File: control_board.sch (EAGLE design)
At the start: 19 parts

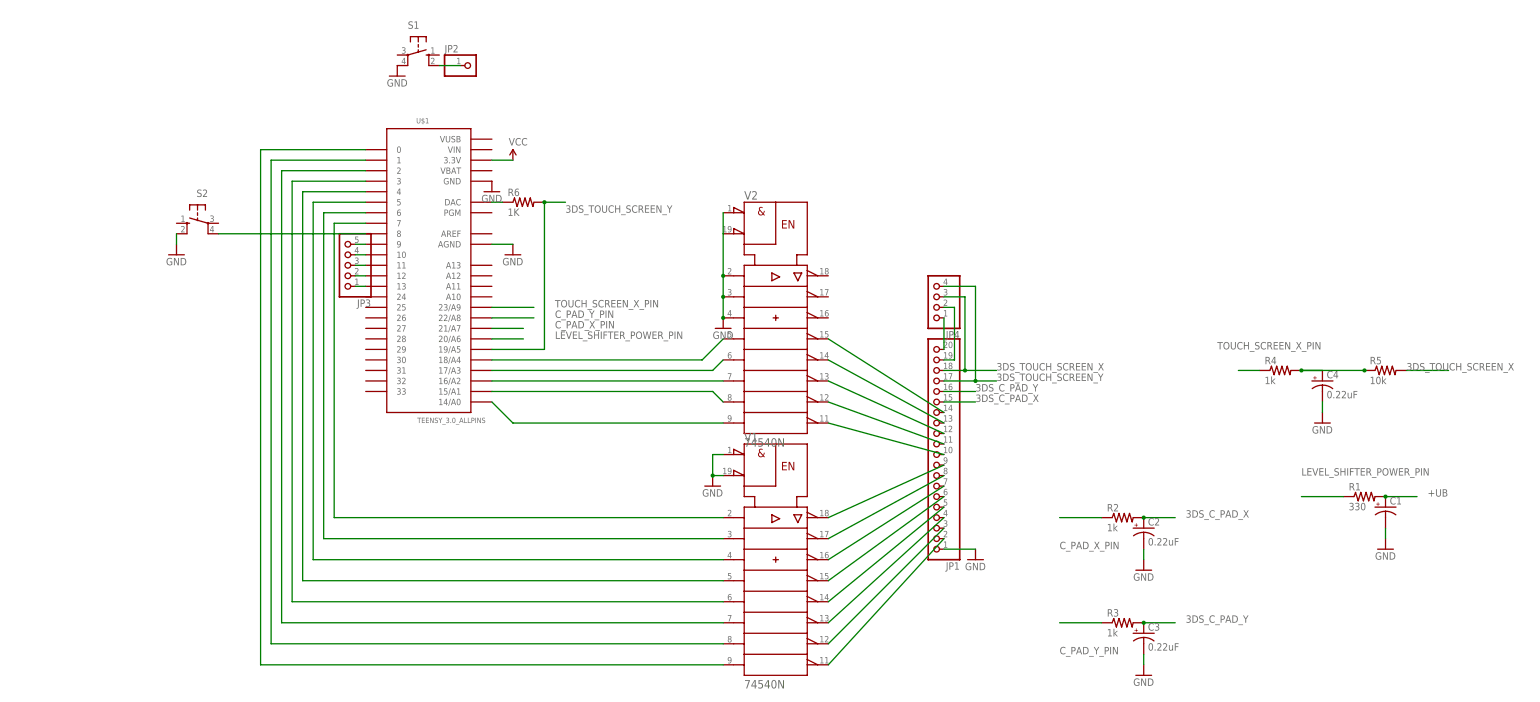
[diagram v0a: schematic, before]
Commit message: First commit
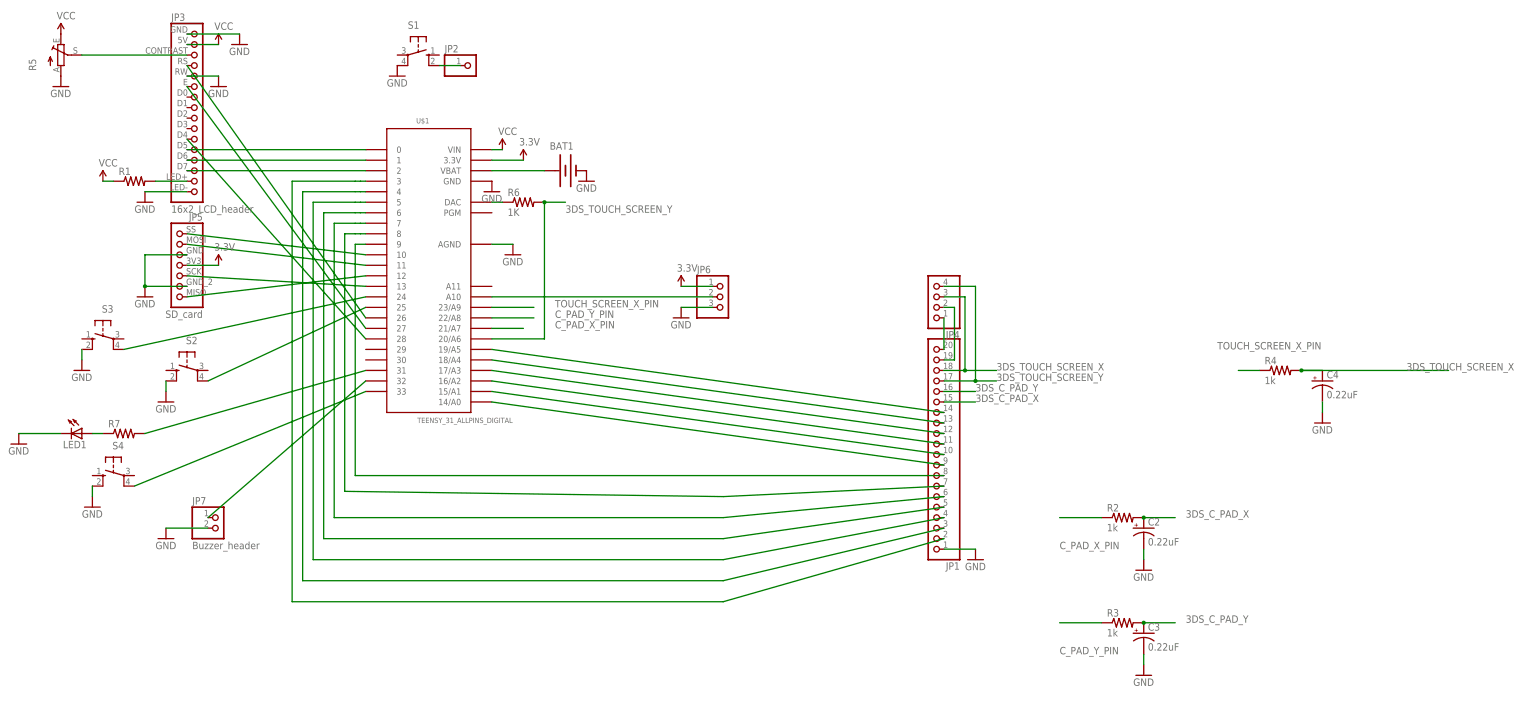
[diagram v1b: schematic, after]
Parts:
- removed C1: (no value), SparkFun-Capacitors:10UF-25V-20%(PTH)
- removed V1, V2: 74540N, 74ttl-din:74540N
- added BAT1: (no value), SparkFun-Electromechanical:BATTERY20PTH
- added JP5: SD_card, sd_header:PINHD-1X7
- added JP6: (no value), pinhead:PINHD-1X3
- added JP7: Buzzer_header, pinhead:PINHD-1X2
- added LED1: (no value), adafruit:LED5MM
- added R7: (no value), SparkFun-Resistors:RESISTOREZ
- added S3, S4: (no value), switch-omron:10-XX
- JP3: value (none) -> 16x2_LCD_header; device pinhead:PINHD-1X5 -> LCD_HEADER:PINHD-1X16
- R1: value 330 -> (none); device resistor:R-US_0207/7 -> SparkFun-Resistors:RESISTOREZ
- R2, R3, R4: device resistor:R-US_0207/7 -> SparkFun-Resistors:RESISTORPTH-1/4W-VERT
- R5: value 10k -> (none); device SparkFun-Resistors:RESISTORPTH-1/4W-VERT -> pot:TRIM_EU-CA6V
- R6: device rcl:R-US_0207/7 -> SparkFun-Resistors:RESISTORPTH-1/4W-VERT
- U$1: value TEENSY_3.0_ALLPINS -> TEENSY_31_ALLPINS_DIGITAL; device Teensy3.0:TEENSY_3.0_ALLPINS -> Teensy3.0:TEENSY_31_ALLPINS_DIGITAL
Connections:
- removed net +UB: C1.+, R1.2
- removed net LEVEL_SHIFTER_POWER_PIN: R1.1, U$1.20/A6
- removed net N0: C4.+, R4.2, R5.1
- new net 3.3V: JP5.4, JP6.1, U$1.3.3V
- new net N$37: JP7.1, U$1.32
- net 3DS_TOUCH_SCREEN_X: now also C4.+, R4.2; no longer R5.2
- net 3DS_TOUCH_SCREEN_Y: now also U$1.20/A6; no longer U$1.19/A5
- net GND: now also BAT1.-, JP3.GND, JP3.LED-, JP3.RW, JP5.3, JP5.6, JP6.3, JP7.2, LED1.C, R5.A, S3.S1, S4.S1; no longer C1.-, V11.!G1, V11.!G2, V21.!G1, V21.!G2, V21.A1, V21.A2, V21.A3
- net N$1: now also JP1.7, U$1.8; no longer JP1.2, V11.Y8
- net N$10: now also JP3.CONTRAST, R5.S; no longer JP1.12, V21.Y6
- net N$11: now also JP5.1, U$1.10; no longer JP1.13, V21.Y5
- net N$12: now also JP5.2, U$1.11; no longer JP1.14, V21.Y4
- net N$13: now also JP5.7, U$1.12; no longer JP1.10, V21.Y8
- net N$15: now also JP5.5, U$1.13; no longer U$1.14/A0, V21.A8
- net N$16: now also JP6.2, U$1.A10; no longer U$1.15/A1, V21.A7
- net N$17: now also JP3.D7, U$1.2; no longer U$1.16/A2, V21.A6
- net N$18: now also JP3.D6, U$1.1; no longer U$1.17/A3, V21.A5
- net N$19: now also JP3.D5; no longer V11.A8
- net N$2: now also JP1.8, U$1.9; no longer JP1.3, V11.Y7
- net N$20: now also JP3.D4, U$1.28; no longer U$1.1, V11.A7
- net N$21: now also JP3.E, U$1.27; no longer U$1.2, V11.A6
- net N$22: now also JP1.2; no longer V11.A5
- net N$23: now also JP1.3; no longer V11.A4
- net N$24: now also JP1.4; no longer V11.A3
- net N$25: now also JP1.5; no longer V11.A2
- net N$26: now also JP1.6; no longer V11.A1
- net N$28: now also JP3.RS, U$1.26; no longer U$1.18/A4, V21.A4
- net N$29: now also BAT1.+, U$1.VBAT; no longer JP3.5, U$1.9
- net N$3: now also JP1.9, U$1.14/A0; no longer JP1.4, V11.Y6
- net N$30: now also S2.P1, U$1.25; no longer JP3.4, U$1.10
- net N$31: now also S3.P1, U$1.24; no longer JP3.3, U$1.11
- net N$32: now also S4.P1, U$1.33; no longer JP3.2, U$1.12
- net N$33: now also R7.2, U$1.31; no longer JP3.1, U$1.13
- net N$36: now also LED1.A, R7.1; no longer S2.P1, U$1.8
- net N$4: now also JP1.10, U$1.15/A1; no longer JP1.5, V11.Y5
- net N$5: now also JP1.11, U$1.16/A2; no longer JP1.6, V11.Y4
- net N$6: now also JP1.12, U$1.17/A3; no longer JP1.7, V11.Y3
- net N$7: now also JP1.13, U$1.18/A4; no longer JP1.8, V11.Y2
- net N$8: now also JP1.14, U$1.19/A5; no longer JP1.9, V11.Y1
- net N$9: now also JP3.LED+, R1.2; no longer JP1.11, V21.Y7
- net VCC: now also JP3.5V, R1.1, R5.E, U$1.VIN; no longer U$1.3.3V
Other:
- moved on the sheet: R1, S2
